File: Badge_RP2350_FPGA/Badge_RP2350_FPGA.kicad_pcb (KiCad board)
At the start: 2 copper layers, 100 x 150 mm, 110 parts, among them J1 USB_C_Receptacle_USB2.0_16P, J2 Conn_01x03_Pin, J3 Conn_01x15_Pin, J4 Conn_01x15_Pin, SW1 SW_Push, SW12 On/Off, SW2 SW_Push, U1 RP2350_60QFN, U2 GW1N-LV9QN88C6_I5_, U3 ME6211C12, U4 TMI7003C, U6 W25Q32JVSS, U7 W25Q32JVSS, Y1 ABM8-272-T3

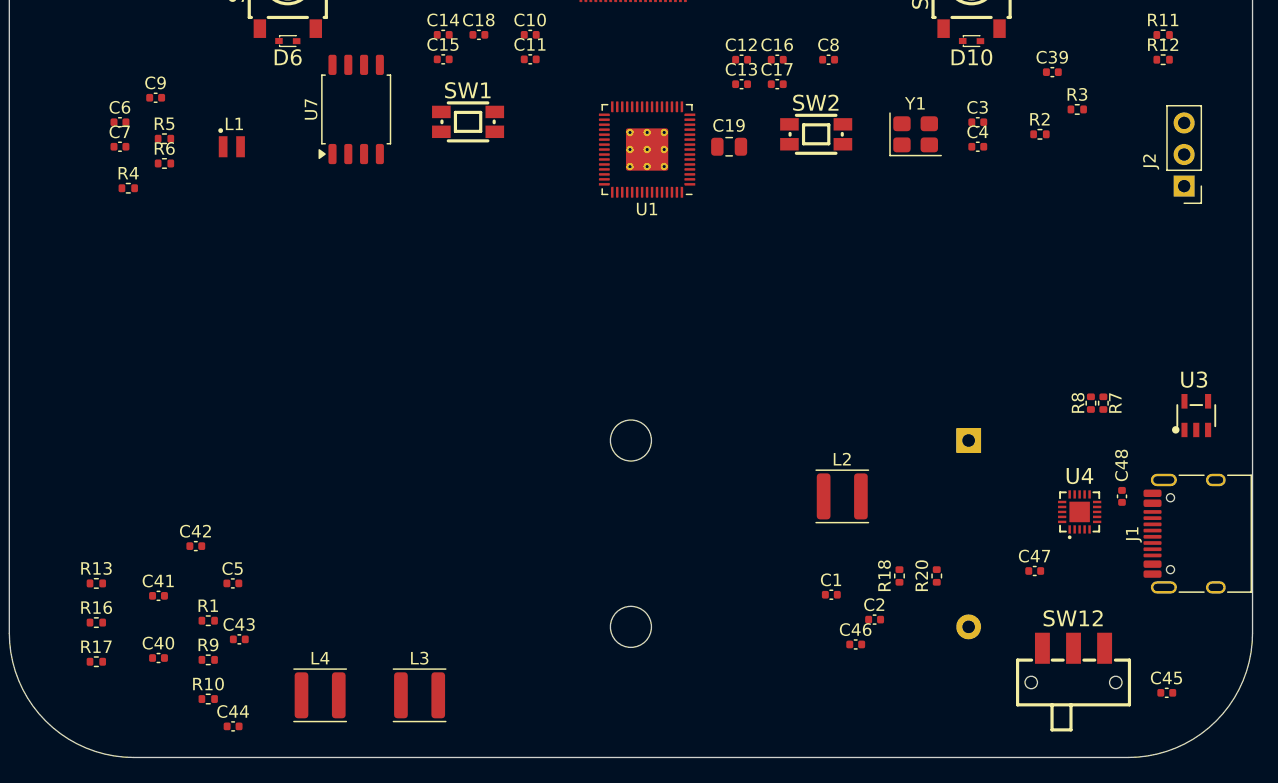
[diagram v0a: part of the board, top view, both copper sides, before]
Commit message: power placement
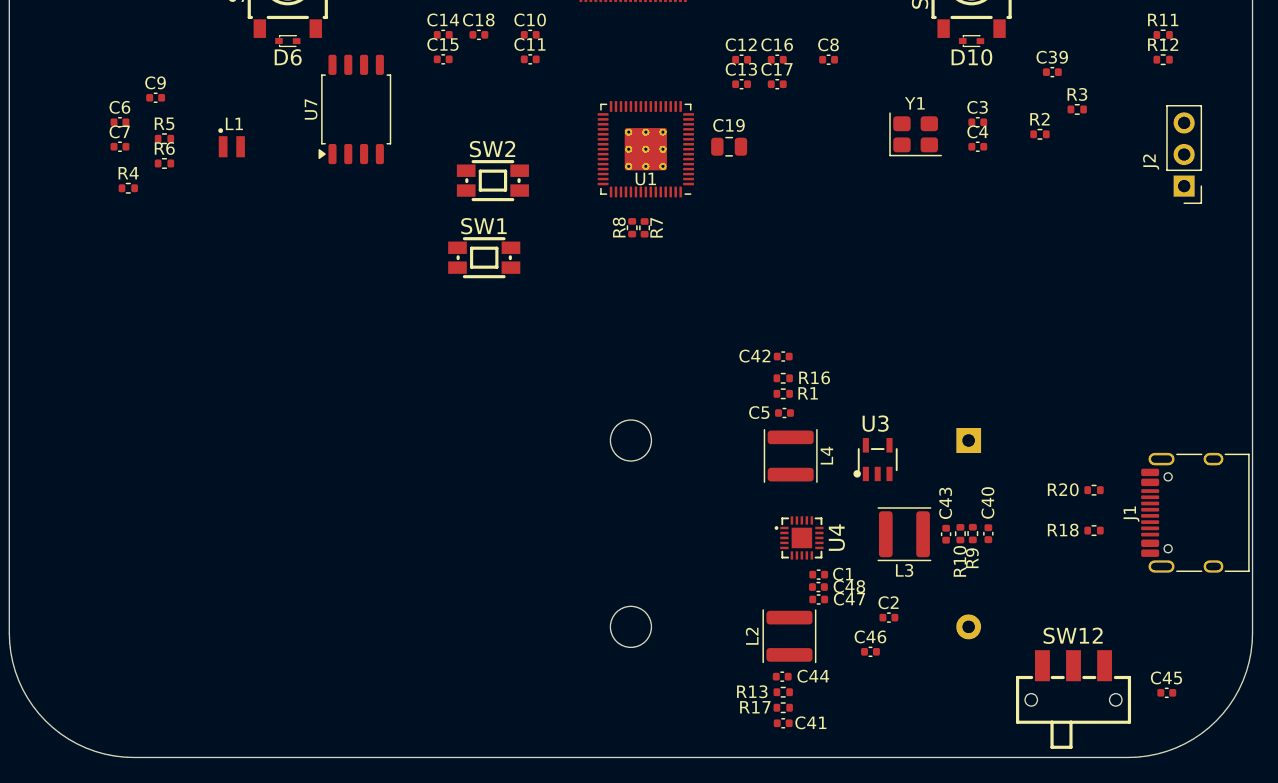
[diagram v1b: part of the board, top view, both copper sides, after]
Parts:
- moved C40 67.5 mm to (128.8, 182.0), turned to -90 degrees
- moved R9 62.3 mm to (127.5, 182.0), turned to 90 degrees
- moved R10 61.9 mm to (126.5, 182.0), turned to 90 degrees
- moved R16 58.6 mm to (112.2, 169.5)
- moved C43 57.5 mm to (125.3, 182.0), turned to 90 degrees
- moved R13 55.9 mm to (112.2, 194.8), turned to 180 degrees
- moved R17 55.4 mm to (112.2, 196.0), turned to 180 degrees
- moved C41 51.3 mm to (112.2, 197.2), turned to 180 degrees
- moved R1 49.7 mm to (112.2, 170.8), turned to 180 degrees
- moved C42 49.7 mm to (112.2, 167.8)
- moved C5 46.4 mm to (112.3, 172.3), turned to 180 degrees
- moved C44 44.4 mm to (112.2, 193.5), turned to 180 degrees
- moved L4 42.5 mm to (112.8, 175.8), turned to -90 degrees
- moved L3 41.1 mm to (122.0, 182.0), turned to 180 degrees
- moved R8 39.5 mm to (100.1, 157.4)
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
